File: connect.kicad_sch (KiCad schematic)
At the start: 35 parts, among them J10 USB_A, J11 Conn_01x02, J9 USB_OTG, U10 AP22653W6-7, U11 TPD4EUSB30, U8 FSUSB42MUX, U9 USB2514B_Bi, Y1 Crystal_Small

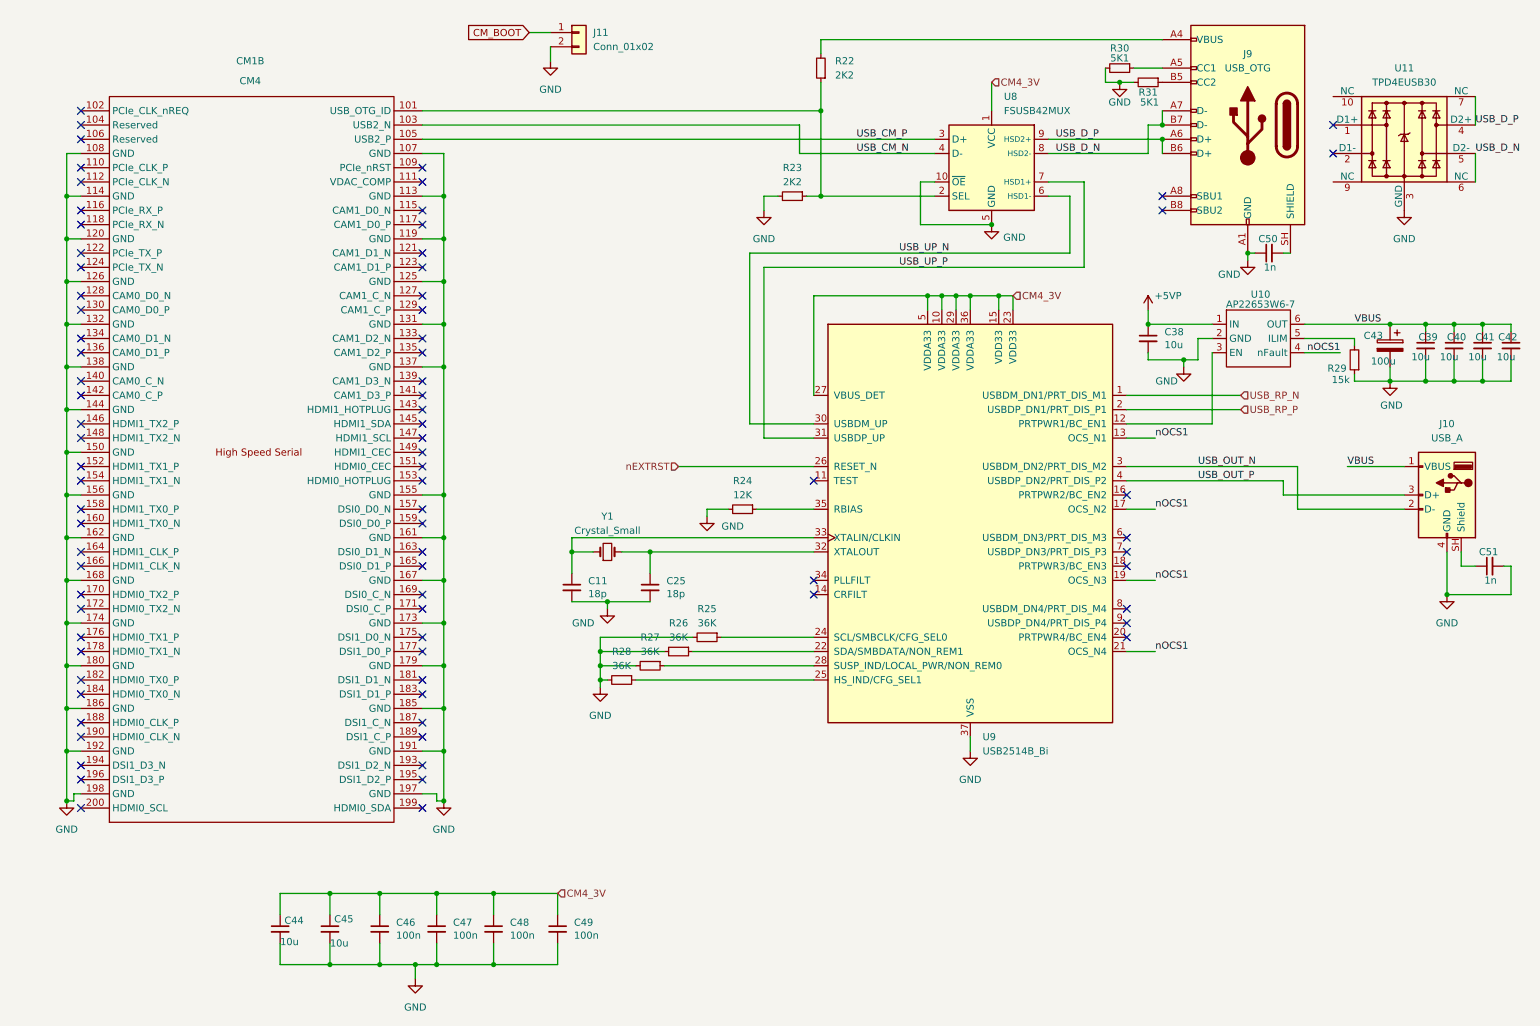
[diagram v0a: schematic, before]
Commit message: Changed to CM5, removed unnecessary USB chips, Changing RP2024 to STM32.
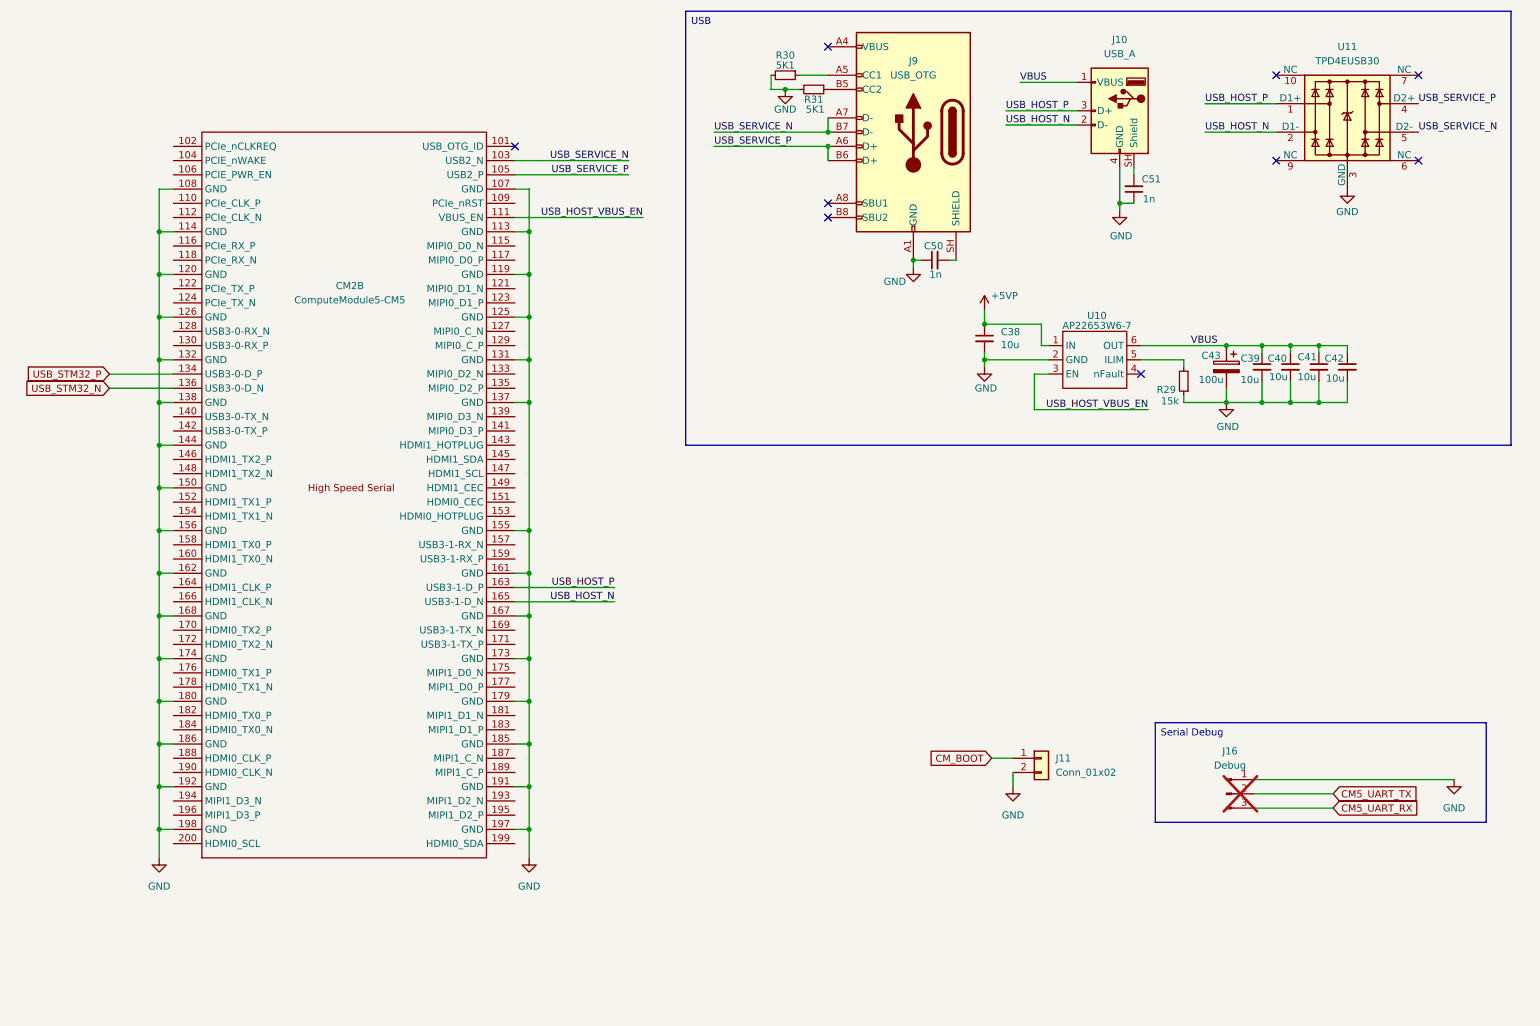
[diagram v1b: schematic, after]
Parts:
- removed C11, C25: 18p, Capacitor_SMD:C_0805_2012Metric, symbol Device:C_Small
- removed C44, C45: 10u, Capacitor_SMD:C_0805_2012Metric, symbol Device:C_Small
- removed C46, C47, C48, C49: 100n, Capacitor_SMD:C_0805_2012Metric, symbol Device:C_Small
- removed CM1: CM4, Pedalboard Library:Raspberry-Pi-4-Compute-Module, symbol pedalboard:CM4
- removed R22, R23: 2K2, Resistor_SMD:R_0805_2012Metric, symbol Device:R_Small
- removed R24: 12K, Resistor_SMD:R_0805_2012Metric, symbol Device:R_Small
- removed R25, R26, R27, R28: 36K, Resistor_SMD:R_0805_2012Metric, symbol Device:R_Small
- removed U8: FSUSB42MUX, Package_SO:TSSOP-10_3x3mm_P0.5mm, symbol Interface_USB:FSUSB42MUX
- removed U9: USB2514B_Bi, Package_DFN_QFN:QFN-36-1EP_6x6mm_P0.5mm_EP3.7x3.7mm, symbol Interface_USB:USB2514B_Bi
- removed Y1: Crystal_Small, Crystal:Crystal_SMD_5032-2Pin_5.0x3.2mm, symbol Device:Crystal_Small
- added CM2: ComputeModule5-CM5, CM5IO:Raspberry-Pi-5-Compute-Module, symbol CM5IO:ComputeModule5-CM5
- added J16: Debug, Connector_PinHeader_2.54mm:PinHeader_1x03_P2.54mm_Vertical, symbol Connector:Conn_01x03_Pin
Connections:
- net USB_OUT_N is gone; now on net USB_HOST_N: J10.2 (D-)
- net USB_OUT_P is gone; now on net USB_HOST_P: J10.3 (D+)
- net GND: now also C51.1, CM2.107 (GND), CM2.108 (GND), CM2.113 (GND), CM2.114 (GND), CM2.119 (GND), CM2.120 (GND), CM2.125 (GND), CM2.126 (GND), CM2.131 (GND), CM2.132 (GND), CM2.137 (GND), CM2.138 (GND), CM2.144 (GND), CM2.150 (GND), CM2.155 (GND), CM2.156 (GND), CM2.161 (GND), CM2.162 (GND), CM2.167 (GND), CM2.168 (GND), CM2.173 (GND), CM2.174 (GND), CM2.179 (GND), CM2.180 (GND), CM2.185 (GND), CM2.186 (GND), CM2.191 (GND), CM2.192 (GND), CM2.197 (GND), CM2.198 (GND), J16.1 (Pin_1); no longer C51.2
- net at J10.SH (Shield): now also C51.2; no longer C51.1
- net USB_HOST_VBUS_EN: now reaches U10.3 (EN)
- net USB_HOST_VBUS_EN: now also CM2.111 (VBUS_EN)
- net USB_HOST_P: now reaches U11.1 (D1+)
- net USB_HOST_P: now also CM2.163 (USB3-1-D_P)
- net USB_HOST_N: now reaches U11.2 (D1-)
- net USB_HOST_N: now also CM2.165 (USB3-1-D_N)
- net USB_D_N renamed USB_SERVICE_N
- net USB_SERVICE_N: now also CM2.103 (USB2_N); no longer U11.6 (NC)
- net USB_D_P renamed USB_SERVICE_P
- net USB_SERVICE_P: now also CM2.105 (USB2_P); no longer U11.7 (NC)
- net nOCS1: no longer names the net of U10.4 (nFault)
- new net CM5_UART_RX: J16.3 (Pin_3)
- new net CM5_UART_TX: J16.2 (Pin_2)
- new net USB_STM32_N: CM2.136 (USB3-0-D_N)
- new net USB_STM32_P: CM2.134 (USB3-0-D_P)
- no-connect marks 81 -> 9
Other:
- moved on the sheet: C38, C39, C40, C41, C42, C43, C50, C51, J10, J11, J9, R29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

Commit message: metadata
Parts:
- R30, R31: Supplier https://www.digikey.ch/de/products/detail/stackpole-electro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 -> (none)
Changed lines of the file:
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@@
 			)
 		)
-		(property "Supplier" "https://www.digikey.ch/de/products/detail/stackpole-electronics-inc/RMCF0805FT2K20/1760345"
+		(property "Supplier" ""
 			(at 157.48 30.48 0)
 			(hide yes)
@@
 			)
 		)
-		(property "Supplier" "https://www.digikey.ch/de/products/detail/stackpole-electronics-inc/RMCF0805FT2K20/1760345"
+		(property "Supplier" ""
 			(at 152.4 27.94 0)
 			(hide yes)
